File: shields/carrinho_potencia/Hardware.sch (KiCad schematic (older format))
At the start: 87 parts, among them J1 Conn_01x02, J10 Conn_01x04, J11 Conn_01x04, J12 Conn_02x13_Odd_Even, J13 Conn_01x02, J14 Conn_01x02, J2 Conn_01x04, J3 Conn_01x02, J4 Conn_01x02_Male, J5 Conn_01x02_Male, J6 Conn_01x02_Male, J7 Conn_01x02_Male, J8 Conn_01x03, J9 Conn_01x03, Q1 BD140, Q10 BC548, Q11 BD139, Q12 BD139, Q2 BD140, Q3 BC548, Q4 BC548, Q5 BD139, Q6 BD139, Q7 BD140, Q8 BD140, Q9 BC548, U1 LM393, U2 TCRT5000, U3 LM324, U4 HC-05, U5 TCRT5000

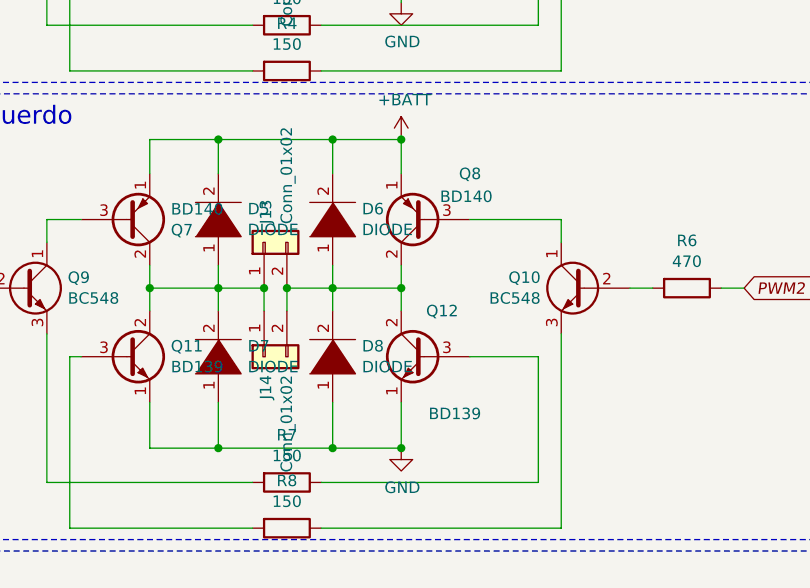
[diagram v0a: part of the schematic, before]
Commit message: Removed backup files
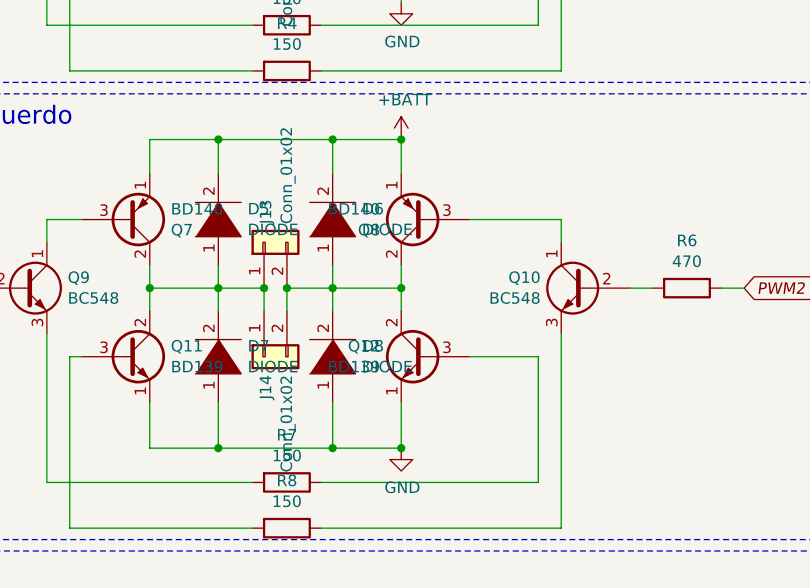
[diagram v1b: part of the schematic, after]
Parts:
- D1, D2, D3, D4, D5, D6, D7, D8: footprint Diode_THT:D_A-405_P2.54mm_Vertical_KathodeUp -> Diode_THT:D_A-405_P2.54mm_Vertical_AnodeUp
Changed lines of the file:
@@
 U 1 1 5CBAC23F
 P 9300 3050
-F 0 "Q8" H 9050 2850 50  0000 L CNN
-F 1 "BD140" H 9000 2950 50  0000 L CNN
+F 0 "Q8" H 9492 3096 50  0000 L CNN
+F 1 "BD140" H 9492 3005 50  0000 L CNN
 F 2 "Package_TO_SOT_THT:TO-126-3_Vertical" H 9500 2975 50  0001 L CIN
 F 3 "http://www.st.com/internet/com/TECHNICAL_RESOURCES/TECHNICAL_LITERATURE/DATASHEET/CD00001225.pdf" H 9300 3050 50  0001 L CNN
@@
 U 1 1 5CBAC24D
 P 9300 3650
-F 0 "Q12" H 9150 3850 50  0000 L CNN
-F 1 "BD139" H 9050 3400 50  0000 L CNN
+F 0 "Q12" H 9492 3696 50  0000 L CNN
+F 1 "BD139" H 9492 3605 50  0000 L CNN
 F 2 "Package_TO_SOT_THT:TO-126-3_Vertical" H 9500 3575 50  0001 L CIN
 F 3 "http://www.st.com/internet/com/TECHNICAL_RESOURCES/TECHNICAL_LITERATURE/DATASHEET/CD00001225.pdf" H 9300 3650 50  0001 L CNN
@@
 F 0 "D7" V 8446 3522 50  0000 R CNN
 F 1 "DIODE" V 8355 3522 50  0000 R CNN
-F 2 "Diode_THT:D_A-405_P2.54mm_Vertical_KathodeUp" H 8400 3650 50  0001 C CNN
+F 2 "Diode_THT:D_A-405_P2.54mm_Vertical_AnodeUp" H 8400 3650 50  0001 C CNN
 F 3 "~" H 8400 3650 50  0001 C CNN
 	1    8400 3650
@@
 F 0 "D3" V 8446 1522 50  0000 R CNN
 F 1 "DIODE" V 8355 1522 50  0000 R CNN
-F 2 "Diode_THT:D_A-405_P2.54mm_Vertical_KathodeUp" H 8400 1650 50  0001 C CNN
+F 2 "Diode_THT:D_A-405_P2.54mm_Vertical_AnodeUp" H 8400 1650 50  0001 C CNN
 F 3 "~" H 8400 1650 50  0001 C CNN
 	1    8400 1650
@@
 F 0 "D4" V 8750 1600 50  0000 R CNN
 F 1 "DIODE" V 8650 1600 50  0000 R CNN
-F 2 "Diode_THT:D_A-405_P2.54mm_Vertical_KathodeUp" H 8900 1650 50  0001 C CNN
+F 2 "Diode_THT:D_A-405_P2.54mm_Vertical_AnodeUp" H 8900 1650 50  0001 C CNN
 F 3 "~" H 8900 1650 50  0001 C CNN
 	1    8900 1650
@@
 F 0 "D2" V 8800 950 50  0000 R CNN
 F 1 "DIODE" V 8700 1000 50  0000 R CNN
-F 2 "Diode_THT:D_A-405_P2.54mm_Vertical_KathodeUp" H 8900 1050 50  0001 C CNN
+F 2 "Diode_THT:D_A-405_P2.54mm_Vertical_AnodeUp" H 8900 1050 50  0001 C CNN
 F 3 "~" H 8900 1050 50  0001 C CNN
 	1    8900 1050
@@
 F 0 "D1" V 8446 922 50  0000 R CNN
 F 1 "DIODE" V 8550 900 50  0000 R CNN
-F 2 "Diode_THT:D_A-405_P2.54mm_Vertical_KathodeUp" H 8400 1050 50  0001 C CNN
+F 2 "Diode_THT:D_A-405_P2.54mm_Vertical_AnodeUp" H 8400 1050 50  0001 C CNN
 F 3 "~" H 8400 1050 50  0001 C CNN
 	1    8400 1050
@@
 F 0 "D5" V 8446 2922 50  0000 R CNN
 F 1 "DIODE" V 8355 2922 50  0000 R CNN
-F 2 "Diode_THT:D_A-405_P2.54mm_Vertical_KathodeUp" H 8400 3050 50  0001 C CNN
+F 2 "Diode_THT:D_A-405_P2.54mm_Vertical_AnodeUp" H 8400 3050 50  0001 C CNN
 F 3 "~" H 8400 3050 50  0001 C CNN
 	1    8400 3050
@@
 F 0 "D6" V 8946 2922 50  0000 R CNN
 F 1 "DIODE" V 8855 2922 50  0000 R CNN
-F 2 "Diode_THT:D_A-405_P2.54mm_Vertical_KathodeUp" H 8900 3050 50  0001 C CNN
+F 2 "Diode_THT:D_A-405_P2.54mm_Vertical_AnodeUp" H 8900 3050 50  0001 C CNN
 F 3 "~" H 8900 3050 50  0001 C CNN
 	1    8900 3050
@@
 F 0 "D8" V 8946 3522 50  0000 R CNN
 F 1 "DIODE" V 8855 3522 50  0000 R CNN
-F 2 "Diode_THT:D_A-405_P2.54mm_Vertical_KathodeUp" H 8900 3650 50  0001 C CNN
+F 2 "Diode_THT:D_A-405_P2.54mm_Vertical_AnodeUp" H 8900 3650 50  0001 C CNN
 F 3 "~" H 8900 3650 50  0001 C CNN
 	1    8900 3650
